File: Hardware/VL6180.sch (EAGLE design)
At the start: 15 parts, among them U1 VL6180, U3 MIC5219 3.3V

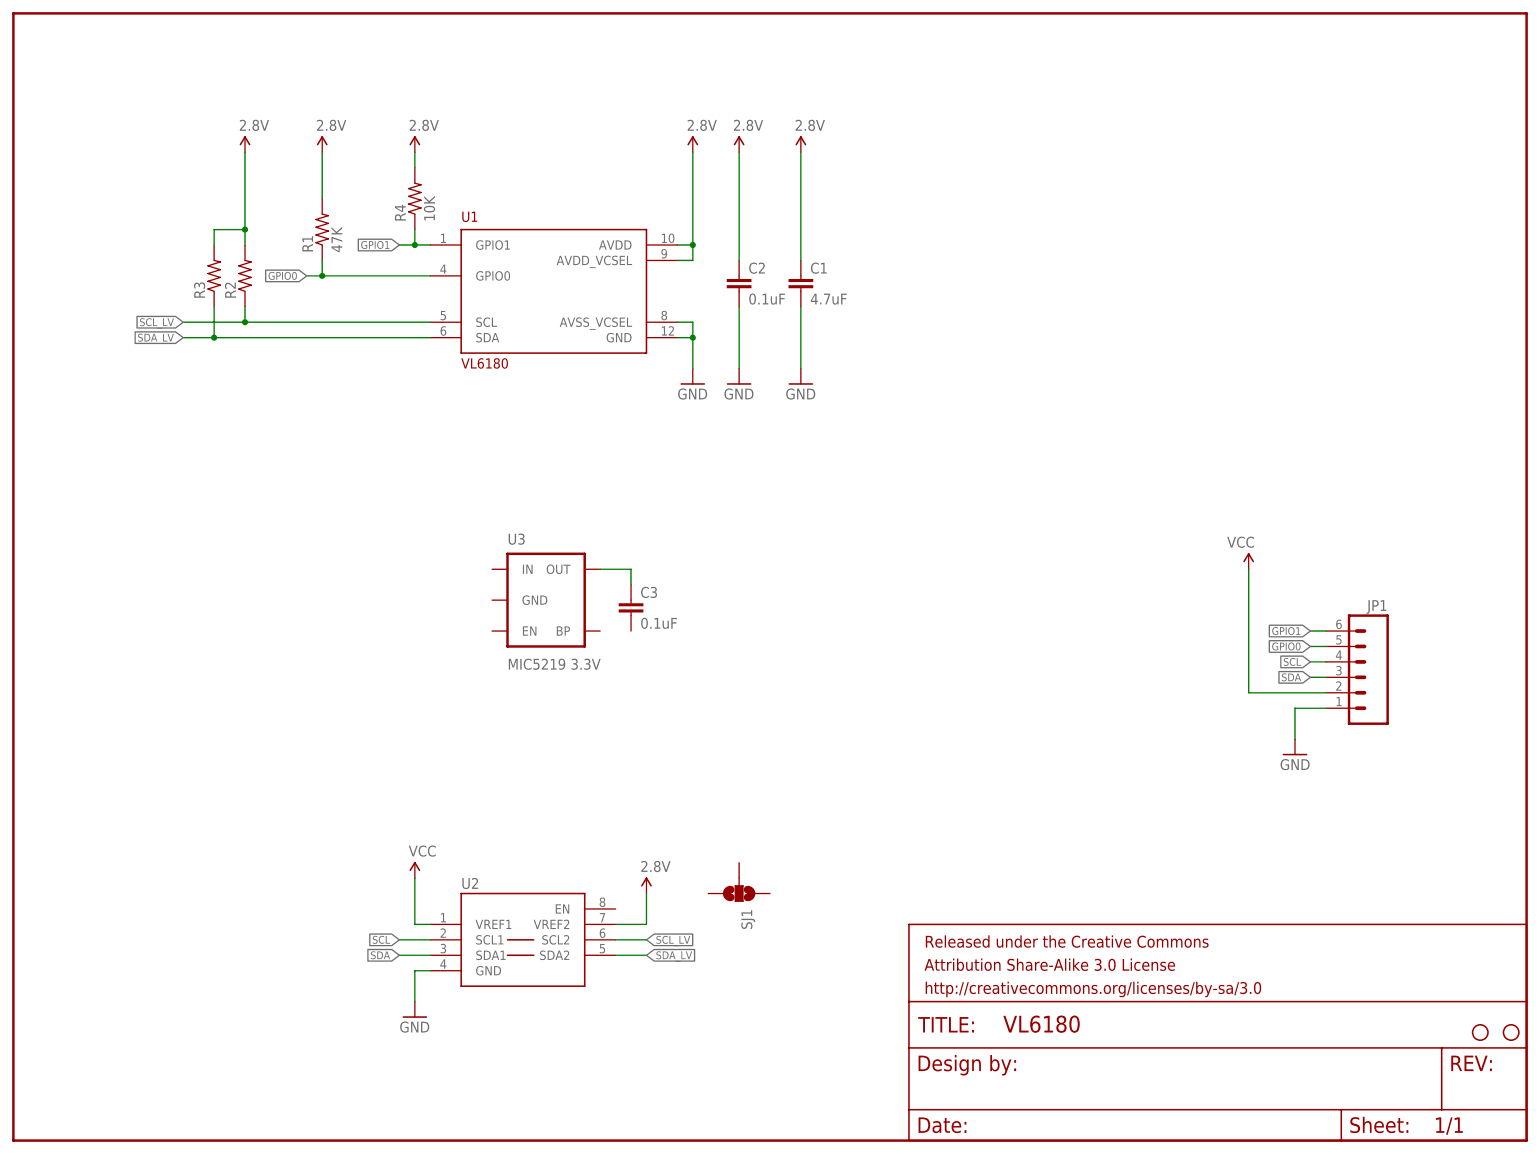
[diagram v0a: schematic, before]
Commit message: Boad Layout finished, looking for review
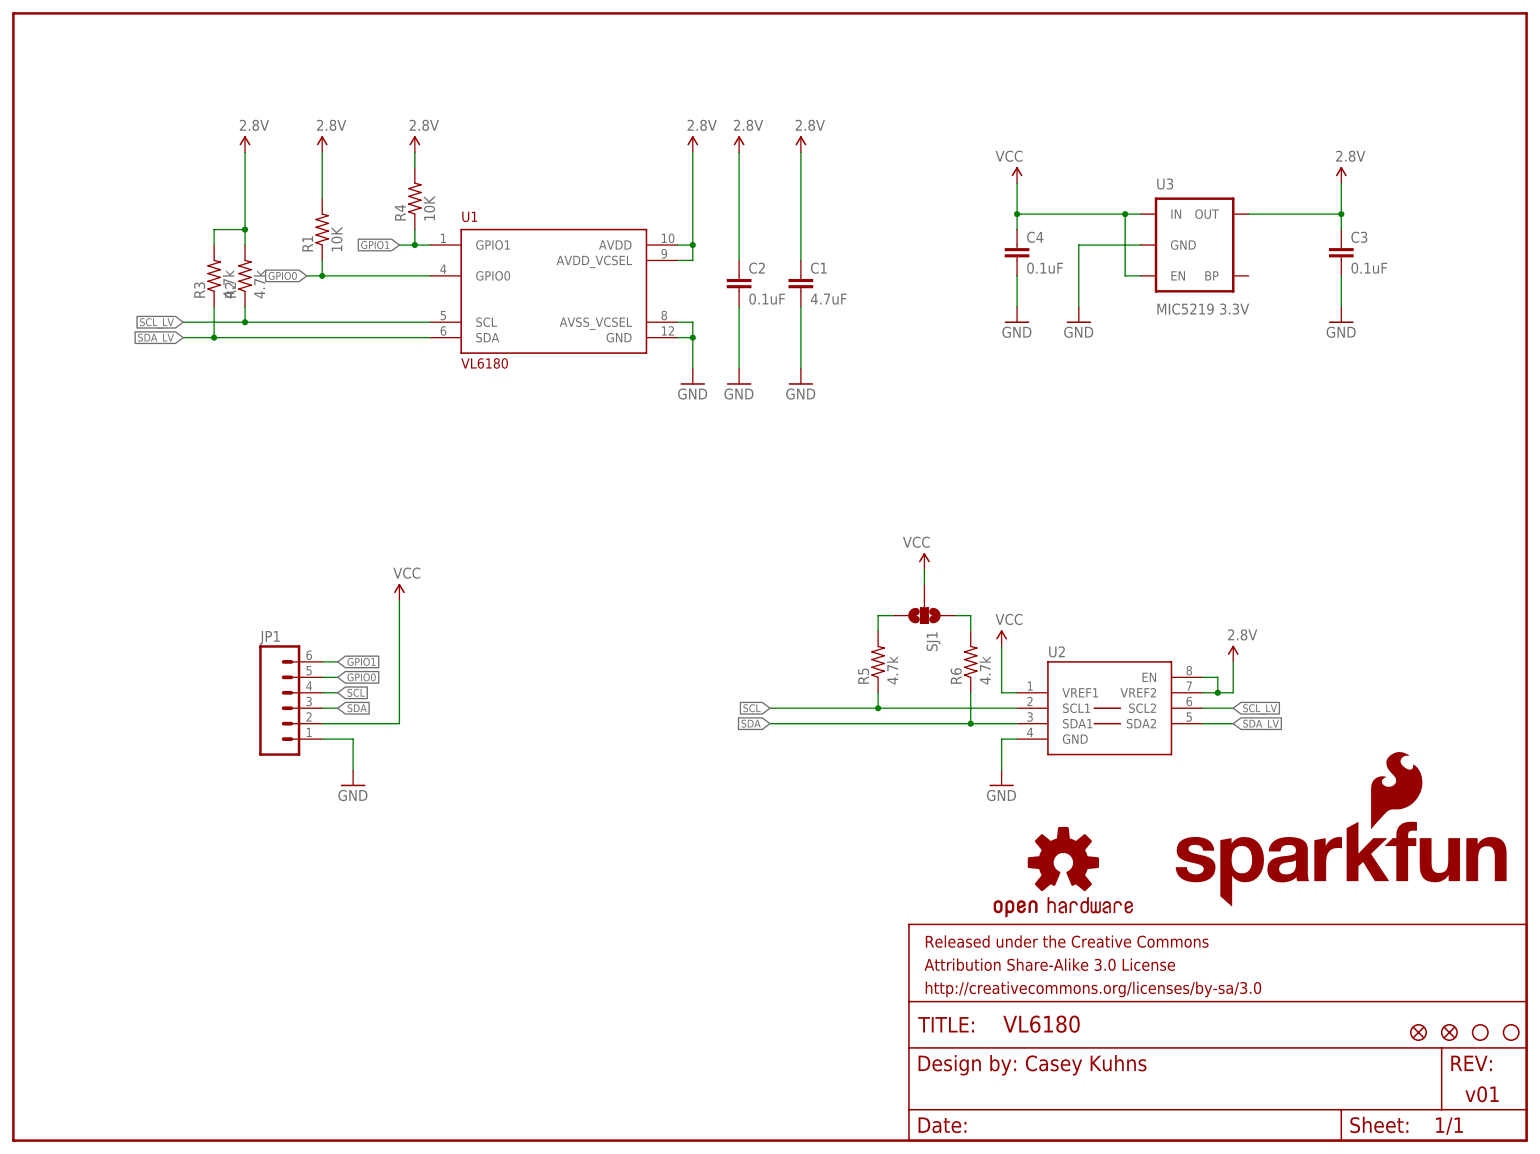
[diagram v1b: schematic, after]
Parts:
- added C4: 0.1uF, SparkFun-Capacitors:0.1UF-25V(+80/-20%)(0603)
- added FID1, FID2: FIDUCIAL1X2, SparkFun-Aesthetics:FIDUCIAL1X2
- added LOGO1: SFE_LOGO_NAME_FLAME.1_INCH, SparkFun-Aesthetics:SFE_LOGO_NAME_FLAME.1_INCH
- added LOGO2: OSHW-LOGOS, SparkFun-Aesthetics:OSHW-LOGOS
- added R5, R6: 4.7k, SparkFun-Resistors:4.7KOHM1/10W1%(0603)
- R1: value 47K -> 10K; device SparkFun-Resistors:47KOHM1/10W1%(0603) -> SparkFun-Resistors:10KOHM1/10W1%(0603)0603
- R2, R3: value (none) -> 4.7k
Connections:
- new net N$3: R5.2, SJ1.3
- net 2.8V: now also C3.1, U2.EN, U3.OUT
- net GND: now also C3.2, C4.2, U3.GND
- net N$2: now also R6.2, SJ1.1; no longer C3.1, U3.OUT
- net SCL: now also R5.1
- net SDA: now also R6.1
- net VCC: now also C4.1, SJ1.2, U3.EN, U3.IN
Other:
- note added: "Casey Kuhns"
- note added: "v01"
- moved on the sheet: C3, JP1, SJ1, U2, U3
